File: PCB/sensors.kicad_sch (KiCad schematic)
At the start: 8 parts, among them IC2 NCP333FCT2G, J3 Conn_Coaxial_Small, J4 Conn_01x03_Socket, U4 LTR-303ALS-01

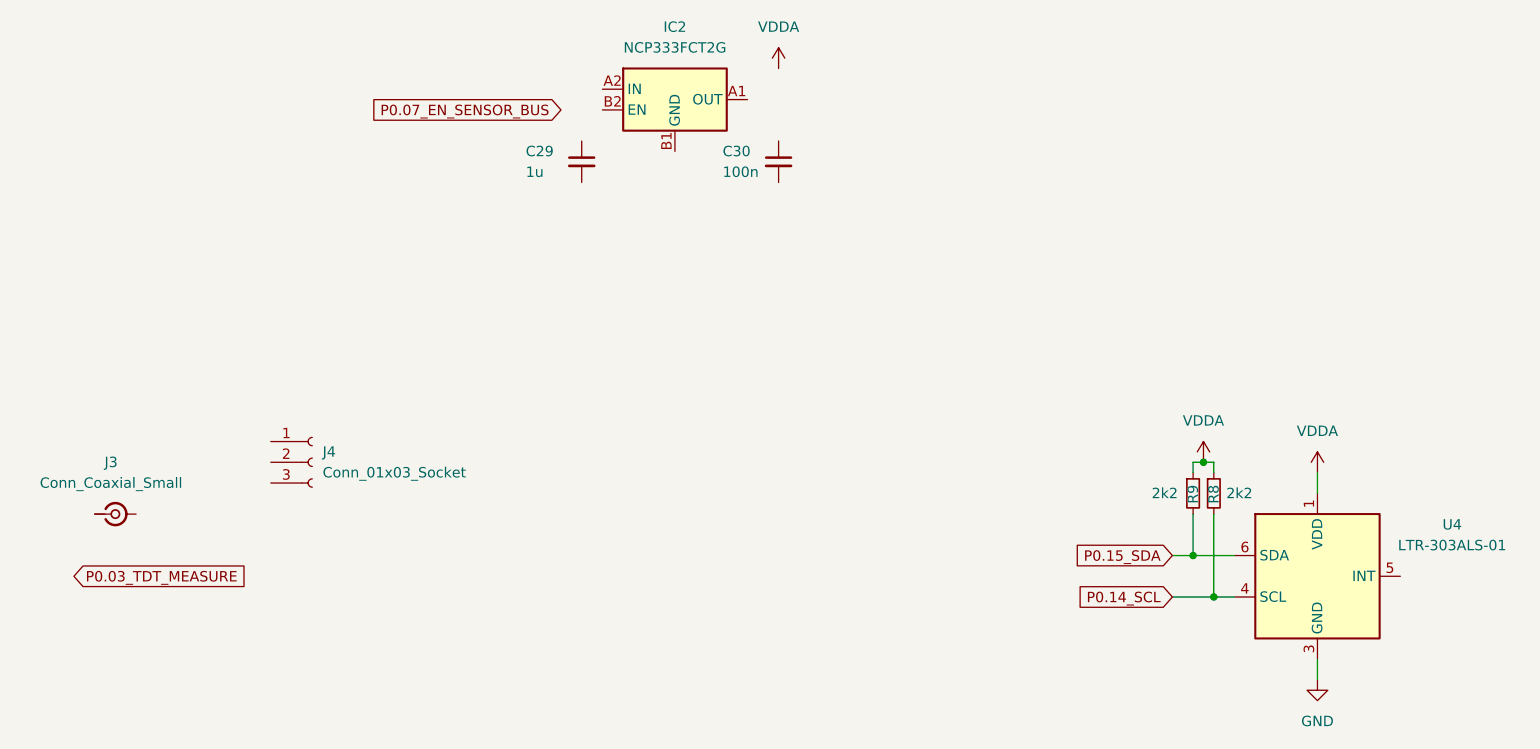
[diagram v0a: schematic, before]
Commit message: Added more Components
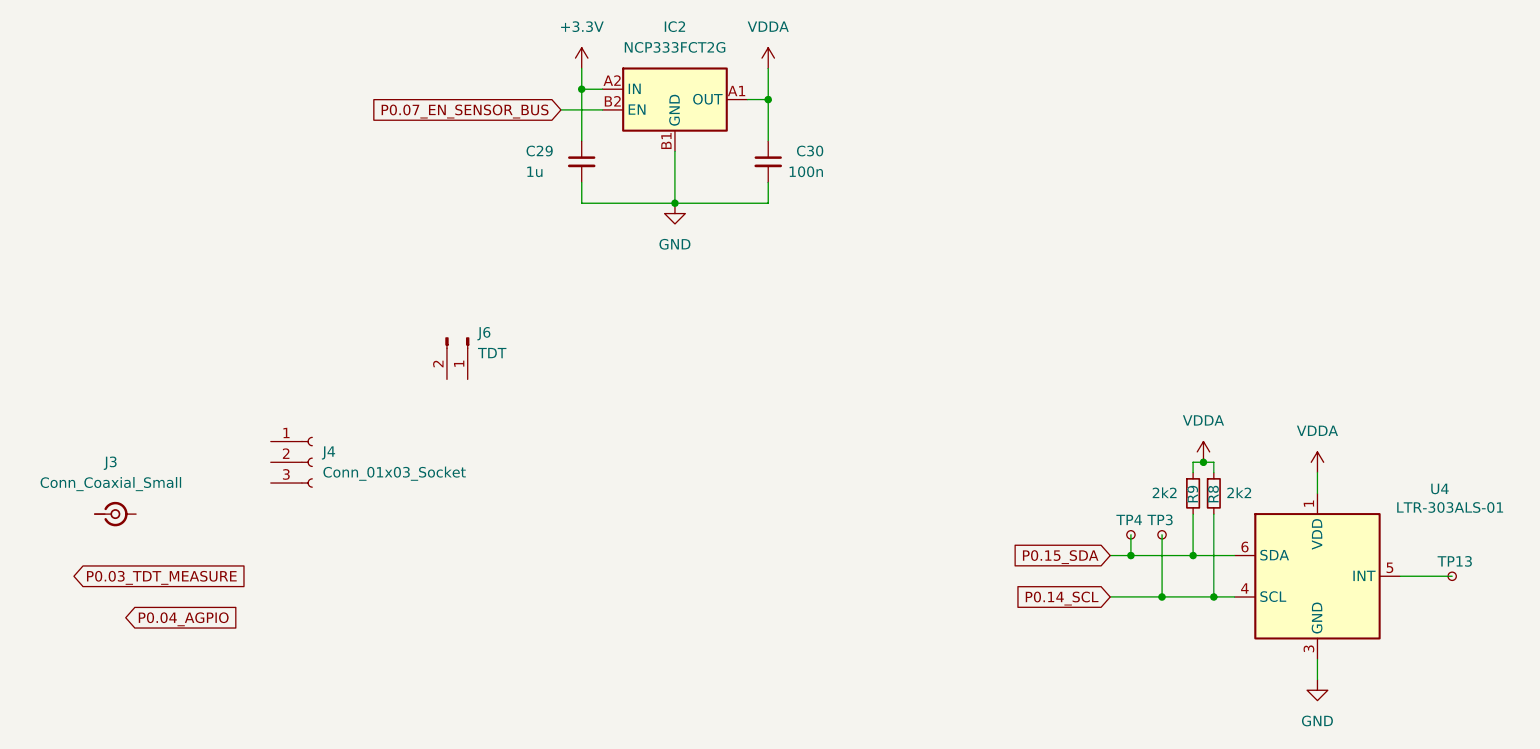
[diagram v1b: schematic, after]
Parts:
- added J6: TDT, Connector_PinHeader_2.54mm:PinHeader_1x02_P2.54mm_Vertical, symbol Connector:Conn_01x02_Pin
- added TP13, TP3, TP4: TestPoint_Small, TestPoint:TestPoint_Pad_D1.0mm, symbol Connector:TestPoint_Small
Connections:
- net GND: now also C29.2, C30.2, IC2.B1 (GND)
- net P0.07_EN_SENSOR_BUS: now also IC2.B2 (EN)
- net P0.14_SCL: now also TP3.1
- net P0.15_SDA: now also TP4.1
- net VDDA: now also C30.1, IC2.A1 (OUT)
- net at U4.5 (INT): now also TP13.1
- net +3.3V: now reaches IC2.A2 (IN)
- net +3.3V: now also C29.1
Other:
- moved on the sheet: C30

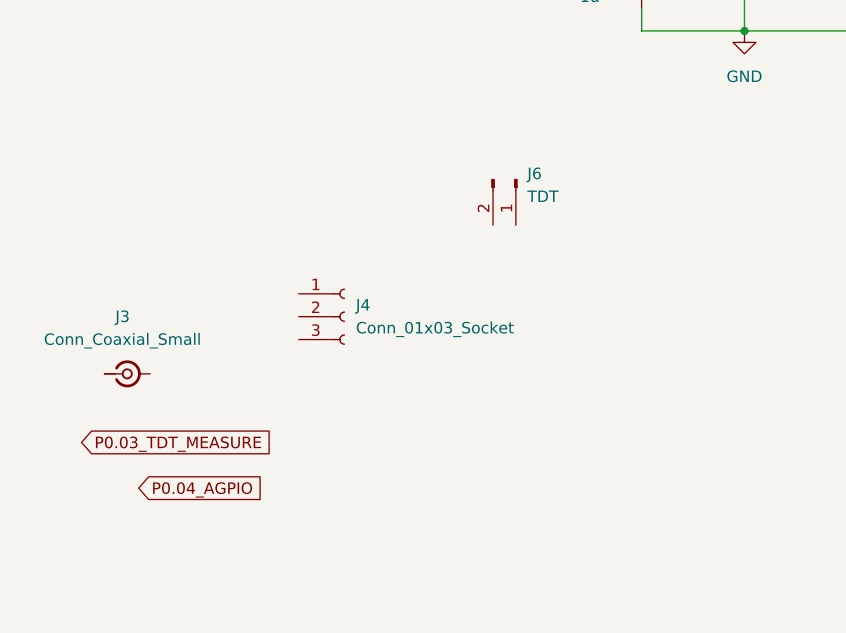
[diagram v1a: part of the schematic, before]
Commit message: Continued on Devboard
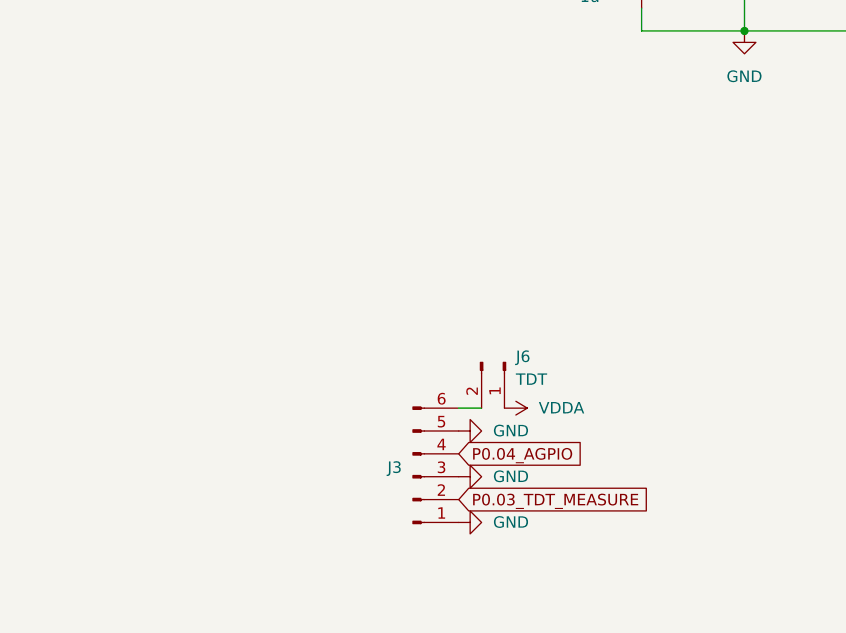
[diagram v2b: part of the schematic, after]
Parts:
- removed J3: Conn_Coaxial_Small, Connector_Coaxial:U.FL_Molex_MCRF_73412-0110_Vertical, symbol Connector:Conn_Coaxial_Small
- removed J4: Conn_01x03_Socket, Connector_PinSocket_2.54mm:PinSocket_1x03_P2.54mm_Horizontal, symbol Connector:Conn_01x03_Socket
- added J3: Conn_01x06_Pin, Connector_PinHeader_2.54mm:PinHeader_1x06_P2.54mm_Vertical, symbol Connector:Conn_01x06_Pin
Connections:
- net GND: now also J3.1 (Pin_1), J3.3 (Pin_3), J3.5 (Pin_5)
- net P0.03_TDT_MEASURE: now also J3.2 (Pin_2)
- net P0.04_AGPIO: now also J3.4 (Pin_4)
- net VDDA: now also J6.1 (Pin_1)
- net at J6.2 (Pin_2): now also J3.6 (Pin_6)
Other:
- moved on the sheet: J6

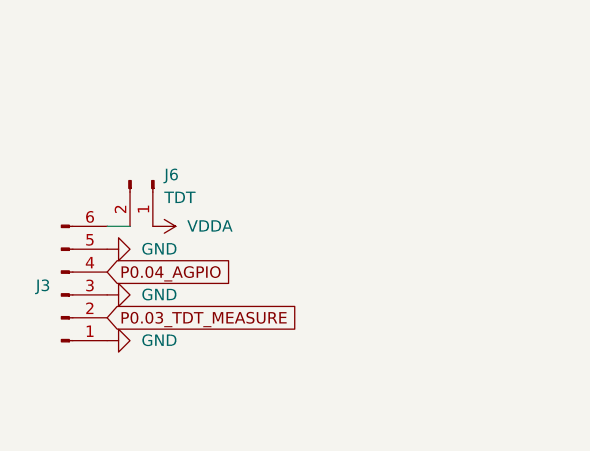
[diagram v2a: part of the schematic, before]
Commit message: Finished Devboard
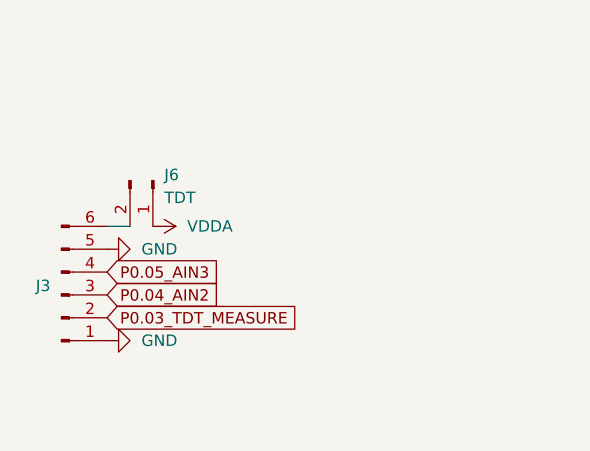
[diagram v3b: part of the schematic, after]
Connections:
- net GND: no longer J3.3 (Pin_3)
- net P0.04_AGPIO renamed P0.05_AIN3
- new net P0.04_AIN2: J3.3 (Pin_3)
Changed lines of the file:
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@@
+		)
+	)
+	(global_label "P0.04_AIN2"
+		(shape input)
+		(at 92.71 95.25 0)
+		(fields_autoplaced yes)
+		(effects
+			(font
+				(size 1.27 1.27)
+			)
+			(justify left)
+		)
+		(property "Intersheetrefs" "${INTERSHEET_REFS}"
+			(at 106.3995 95.25 0)
+			(effects
+				(font
+					(size 1.27 1.27)
+				)
+				(justify left)
+				(hide yes)
+			)
 		)
 	)
@@
 		)
 	)
-	(global_label "P0.04_AGPIO"
+	(global_label "P0.05_AIN3"
 		(shape input)
 		(at 92.71 92.71 0)
@@
 		)
 		(property "Intersheetrefs" "${INTERSHEET_REFS}"
-			(at 107.73 92.71 0)
+			(at 106.3995 92.71 0)
 			(effects
 				(font
@@
 					(unit 1)
 				)
-			)
-		)
-	)
-	(symbol
-		(lib_id "power:GND")
-		(at 92.71 95.25 90)
-		(mirror x)
-		(unit 1)
-		(exclude_from_sim no)
-		(in_bom yes)
-		(on_board yes)
-		(dnp no)
-		(fields_autoplaced yes)
-		(property "Reference" "#PWR070"
-			(at 99.06 95.25 0)
-			(effects
-				(font
-					(size 1.27 1.27)
-				)
-				(hide yes)
-			)
-		)
-		(property "Value" "GND"
-			(at 96.52 95.2501 90)
-			(effects
-				(font
-					(size 1.27 1.27)
-				)
-				(justify right)
-			)
-		)
-		(property "Footprint" ""
-			(at 92.71 95.25 0)
-			(effects
-				(font
-					(size 1.27 1.27)
-				)
-				(hide yes)
-			)
-		)
-		(property "Datasheet" ""
-			(at 92.71 95.25 0)
-			(effects
-				(font
-					(size 1.27 1.27)
-				)
-				(hide yes)
-			)
-		)
-		(property "Description" "Power symbol creates a global label with name \"GND\" , ground"
-			(at 92.71 95.25 0)
-			(effects
-				(font
-					(size 1.27 1.27)
-				)
-				(hide yes)
-			)
-		)
-		(pin "1"
-		)
-		(instances
-			(project "Plant_Thing"
-				(path "/3604ffe7-6852-4862-a71a-75c04c0147cb/38766e62-e2f9-438f-aa7f-b6d1382d0577"
-					(reference "#PWR070")
-					(unit 1)
-				)
